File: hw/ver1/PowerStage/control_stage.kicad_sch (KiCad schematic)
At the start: 55 parts, among them J10 SWD Debug, J11 BMS_Serial, J8 FanConnector, P1 USB_C_Plug_USB2.0, SW3 Boot, SW4 Reset, U10 RP2040, U20 W25Q32JVZP, U21 LM1117MP-5.0, U4 LM1117MP-3.3, Y1 12MHz

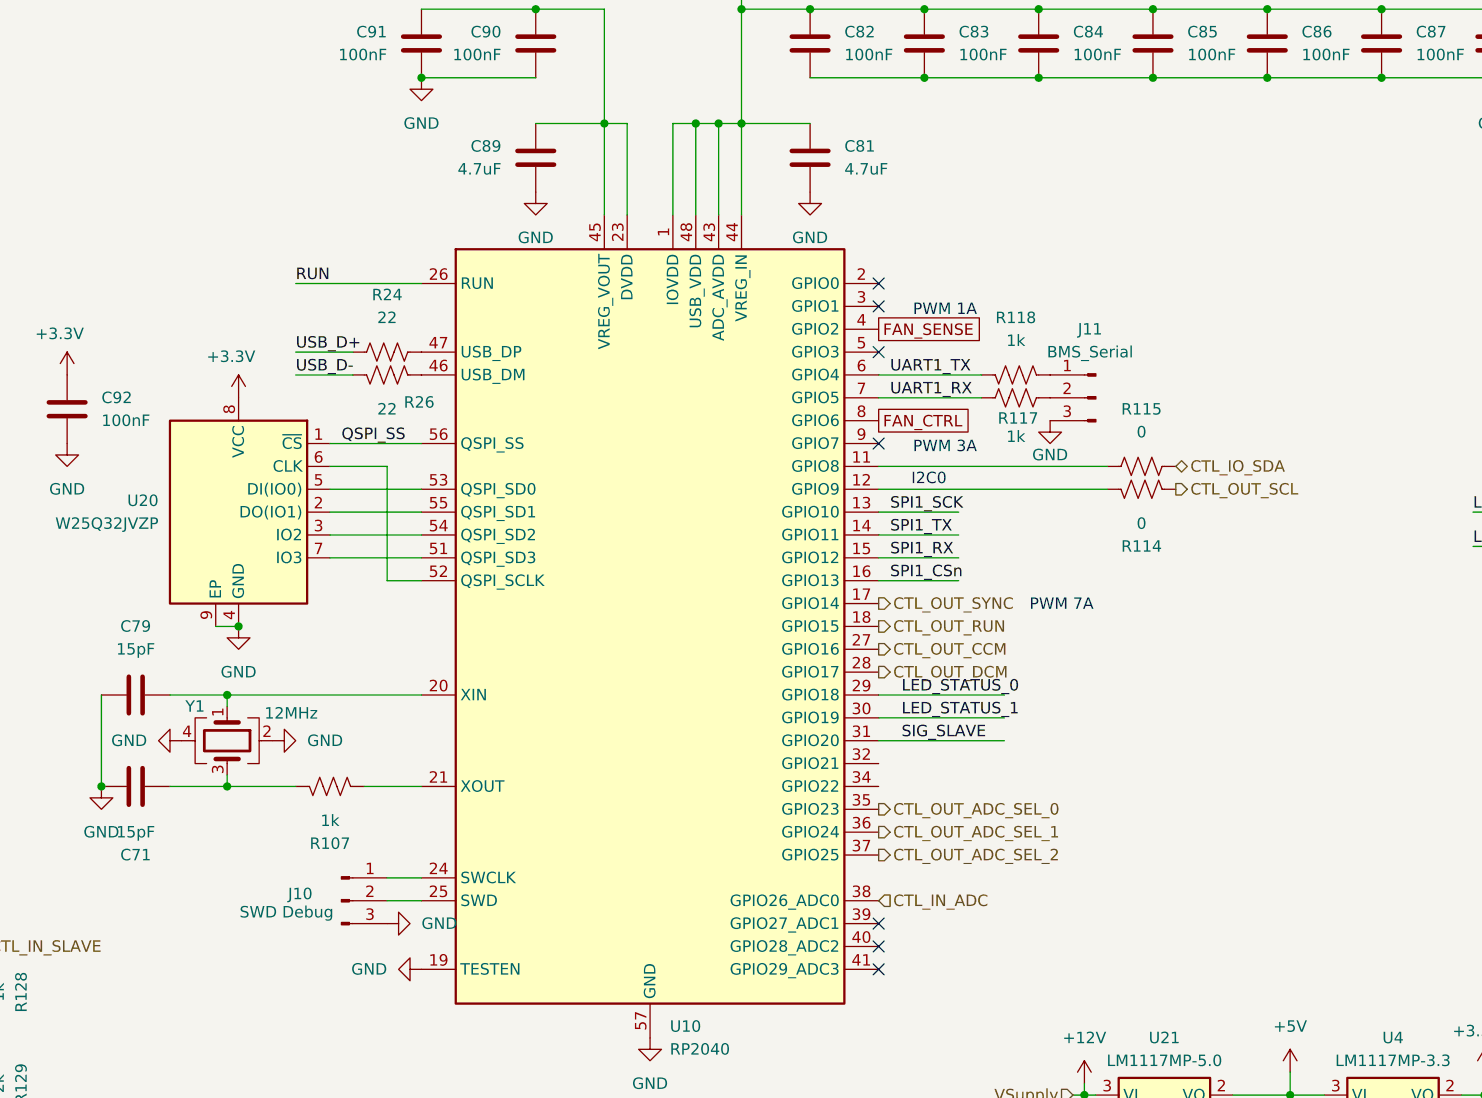
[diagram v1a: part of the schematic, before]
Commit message: Sync work
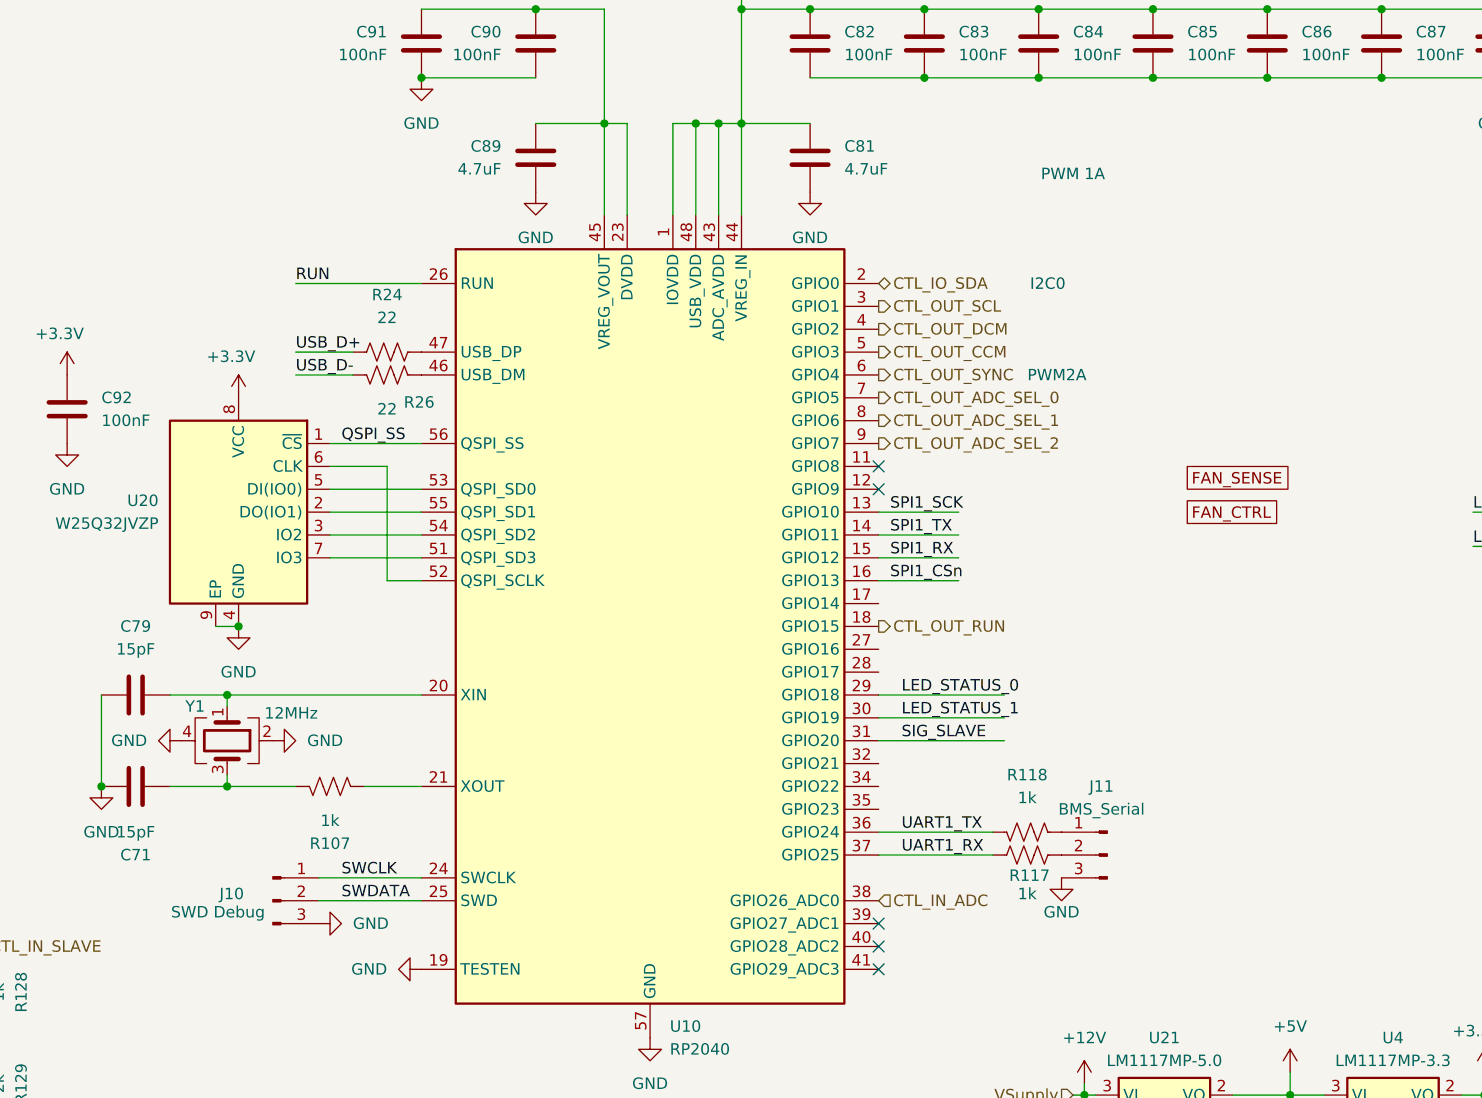
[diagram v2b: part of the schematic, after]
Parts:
- removed R114, R115: 0, Resistor_SMD:R_0603_1608Metric, symbol Device:R_US
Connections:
- net CTL_IO_SDA: now also U10.2 (GPIO0)
- net CTL_OUT_ADC_SEL_0: now also U10.7 (GPIO5); no longer U10.35 (GPIO23)
- net CTL_OUT_ADC_SEL_1: now also U10.8 (GPIO6); no longer U10.36 (GPIO24)
- net CTL_OUT_ADC_SEL_2: now also U10.9 (GPIO7); no longer U10.37 (GPIO25)
- net CTL_OUT_CCM: now also U10.5 (GPIO3); no longer U10.27 (GPIO16)
- net CTL_OUT_DCM: now also U10.4 (GPIO2); no longer U10.28 (GPIO17)
- net CTL_OUT_SCL: now also U10.3 (GPIO1)
- net CTL_OUT_SYNC: now also U10.6 (GPIO4); no longer U10.17 (GPIO14)
- net FAN_CTRL: no longer U10.8 (GPIO6)
- net FAN_SENSE: no longer U10.4 (GPIO2)
- net UART1_RX: now also U10.37 (GPIO25); no longer U10.7 (GPIO5)
- net UART1_TX: now also U10.36 (GPIO24); no longer U10.6 (GPIO4)
- net SWCLK: now reaches J10.1 (Pin_1), U10.24 (SWCLK)
- net SWDATA: now reaches J10.2 (Pin_2), U10.25 (SWD)
- no-connect marks 9 -> 7
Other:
- note added: "PWM2A"
- note removed: "PWM 3A"
- note removed: "PWM 7A"
- moved on the sheet: J10, J11, R117, R118
